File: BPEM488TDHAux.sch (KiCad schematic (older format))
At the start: 100 parts, among them J1 Conn_01x02, J2 Conn_02x18_Odd_Even, J3 DB15_Female, J4 DB15_Female, Q1 ZTX450, Q10 ZTX450, Q11 ZTX450, Q12 ZTX450, Q13 ZTX450, Q14 ZTX450, Q15 ZTX450, Q16 ZTX450, Q17 ZTX450, Q18 ZTX450, Q19 ZTX450, Q2 ZTX450, Q20 ZTX450, Q21 ZTX450, Q22 ZTX450, Q23 ZTX450, Q24 ZTX450, Q25 ZTX450, Q3 ZTX450, Q4 ZTX450, Q5 ZTX450, Q6 ZTX450, Q7 ZTX450, Q8 ZTX450, Q9 ZTX450, U1 LD1085V50, U2 L7808ABV

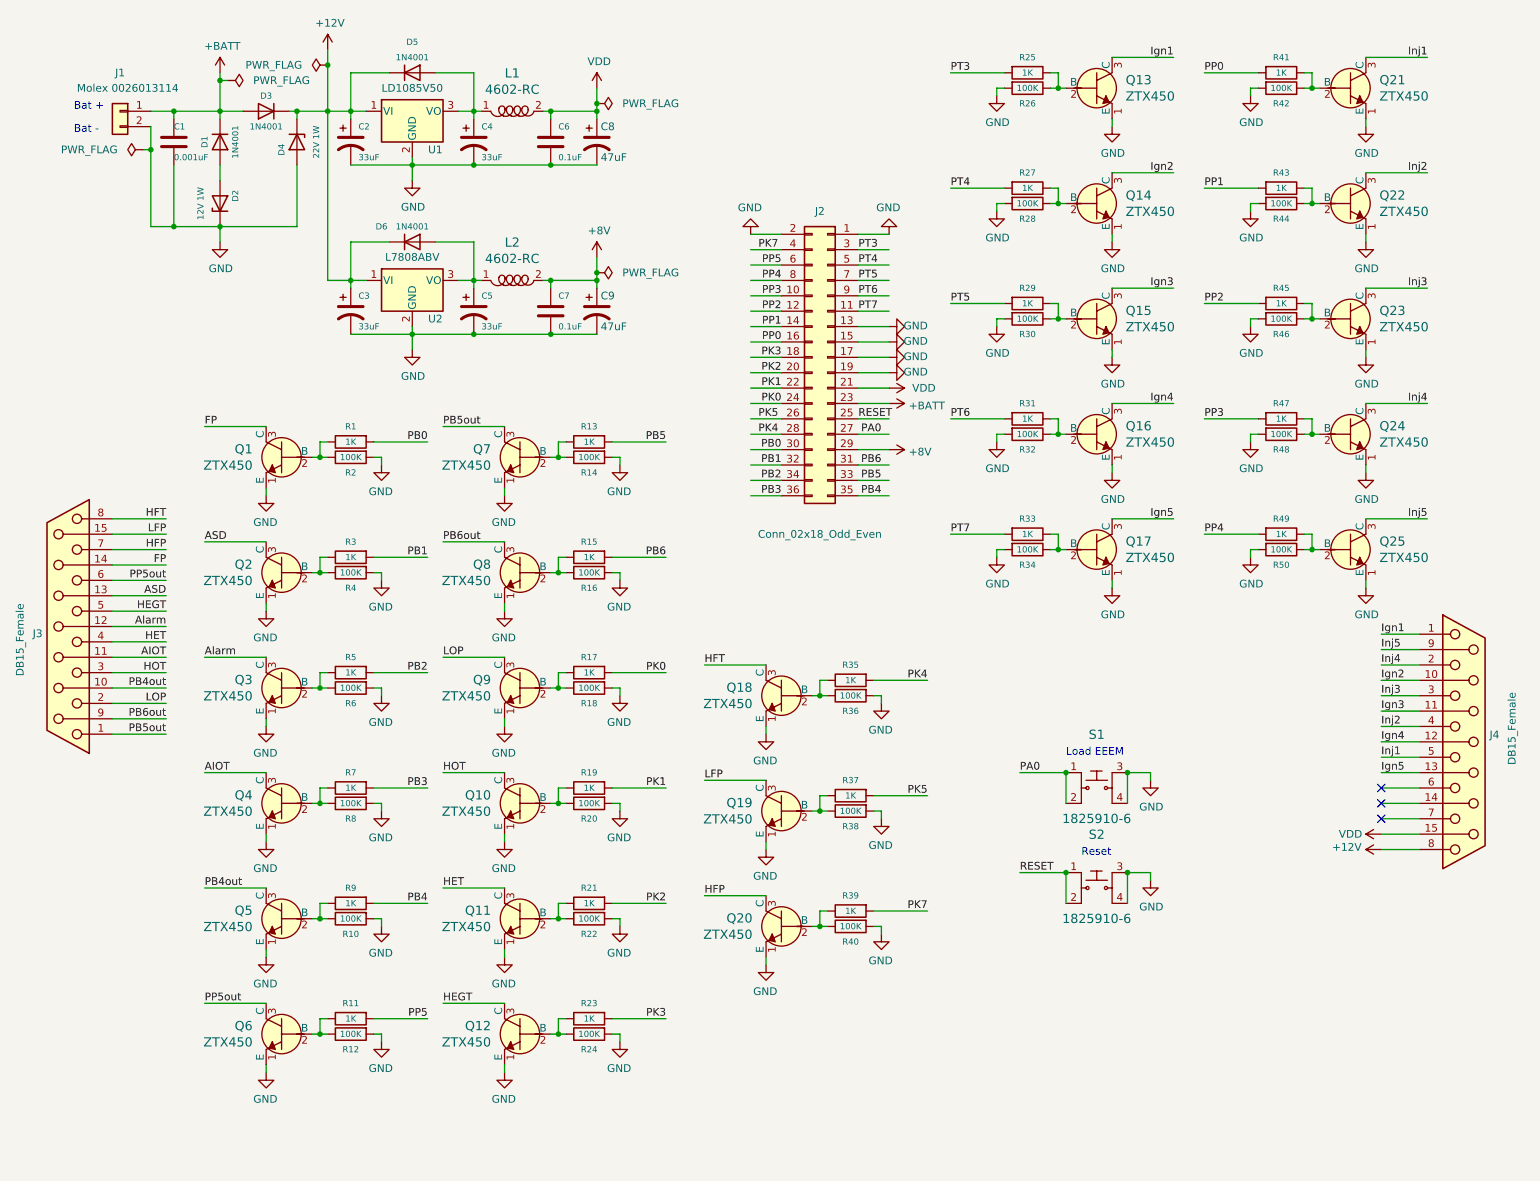
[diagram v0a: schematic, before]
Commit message: Add files via upload
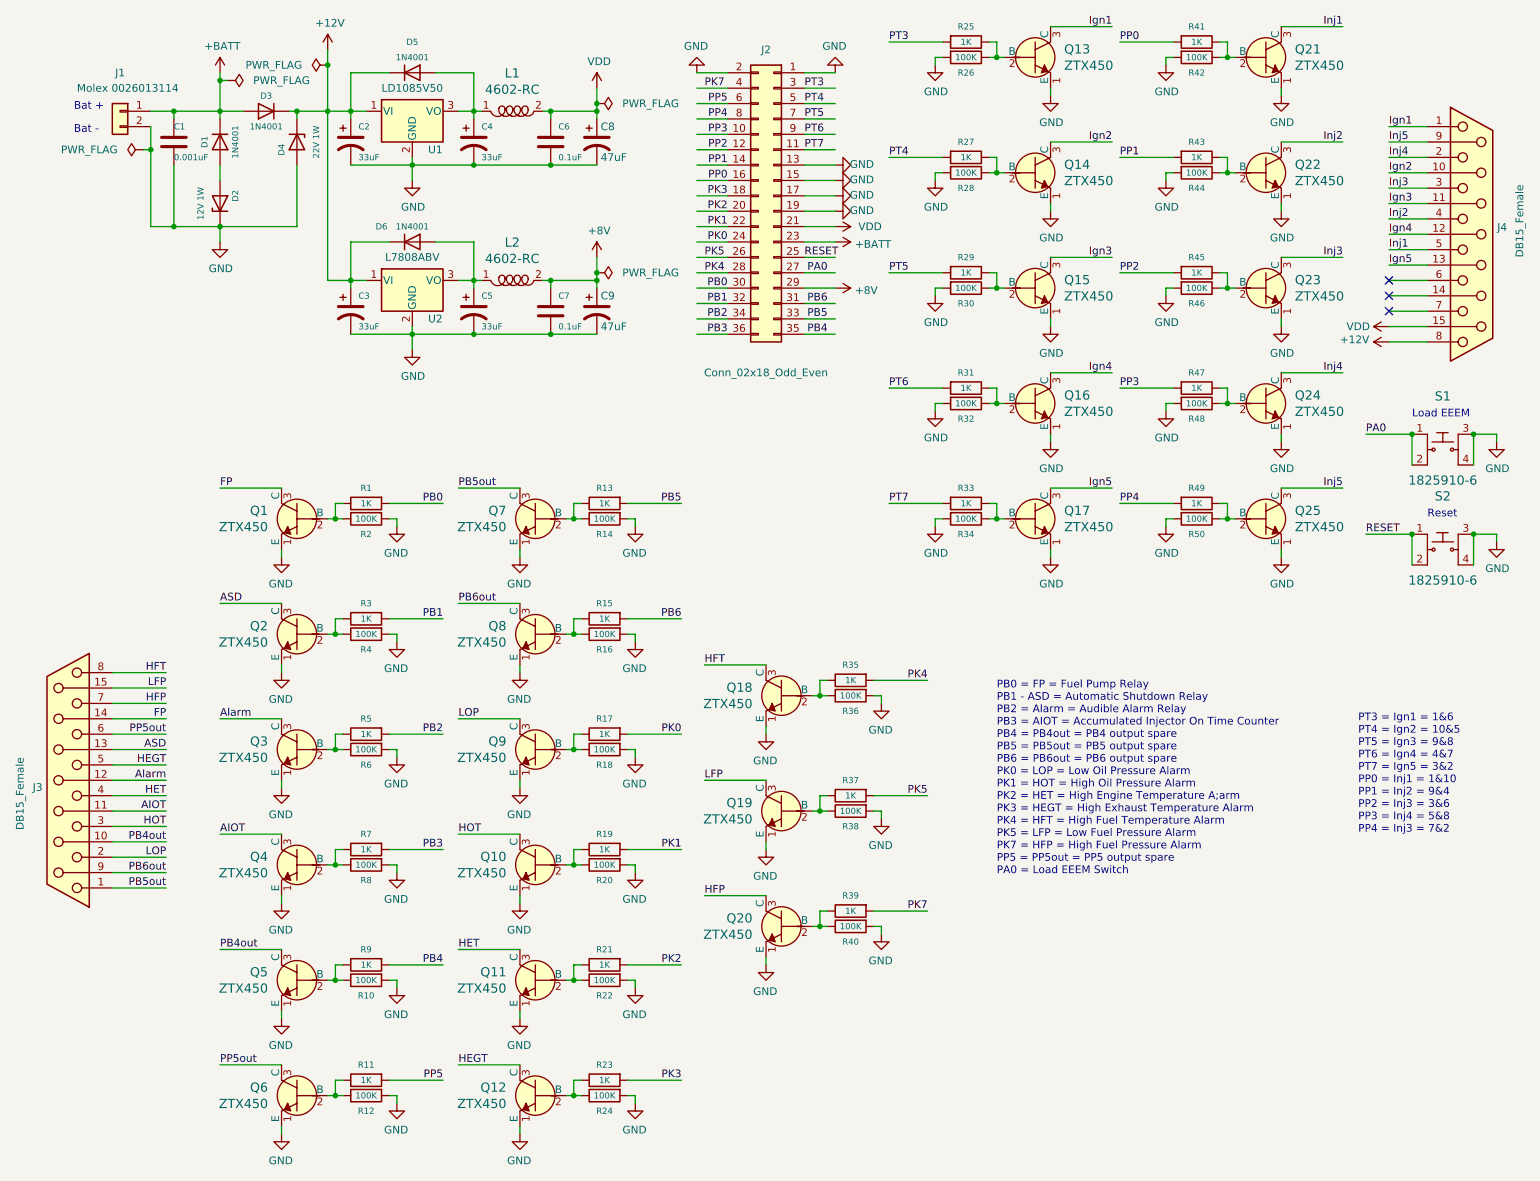
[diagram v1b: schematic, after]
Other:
- note added: "PB0 = FP = Fuel Pump Relay\nPB1 - ASD = Automatic Shutdown Relay\nPB2 = Alarm = Audible Alarm Relay\nPB3 = AIOT = Accumulated Injector On Time Counter\nPB4 = PB4out = PB4 output spare\nPB5 = PB5out = PB5 output spare\nPB6 = PB6out = PB6 output spare\nPK0 = LOP = Low Oil Pressure Alarm\nPK1 = HOT = High Oil Pressure Alarm\nPK2 = HET = High Engine Temperature A;arm\nPK3 = HEGT = High Exhaust Temper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"
- note added: "PT3 = Ign1 = 1&6\nPT4 = Ign2 = 10&5\nPT5 = Ign3 = 9&8\nPT6 = Ign4 = 4&7\nPT7 = Ign5 = 3&2\nPP0 = Inj1 = 1&10\nPP1 = Inj2 = 9&4\nPP2 = Inj3 = 3&6\nPP3 = Inj4 = 5&8\nPP4 = Inj3 = 7&2"
- moved on the sheet: J2, J3, J4, Q1, Q10, Q11, Q12, Q13, Q14, Q15, Q16, Q17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
